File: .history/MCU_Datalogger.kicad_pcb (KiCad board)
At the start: 2 copper layers, 29 parts, among them J1 Conn_01x04_Pin, J2 Conn_01x04_Pin, J3 Conn_01x09_Pin, J4 Conn_02x03_Odd_Even, U1 24LC1025, U2 24LC1025, U3 DS1337S_, U4 ATMEGA328P-AU, Y1 32.768 KHz, Y2 16 MHz

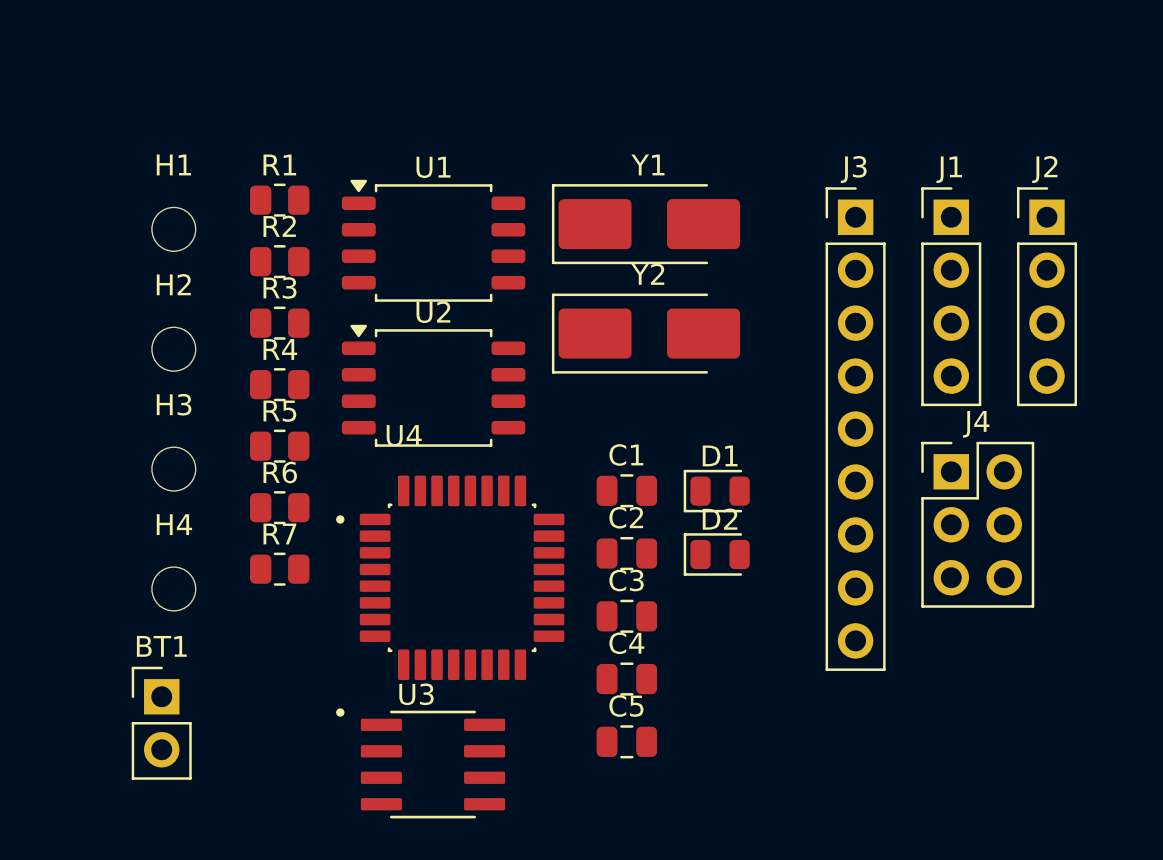
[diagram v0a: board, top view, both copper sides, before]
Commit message: footprint placement completed
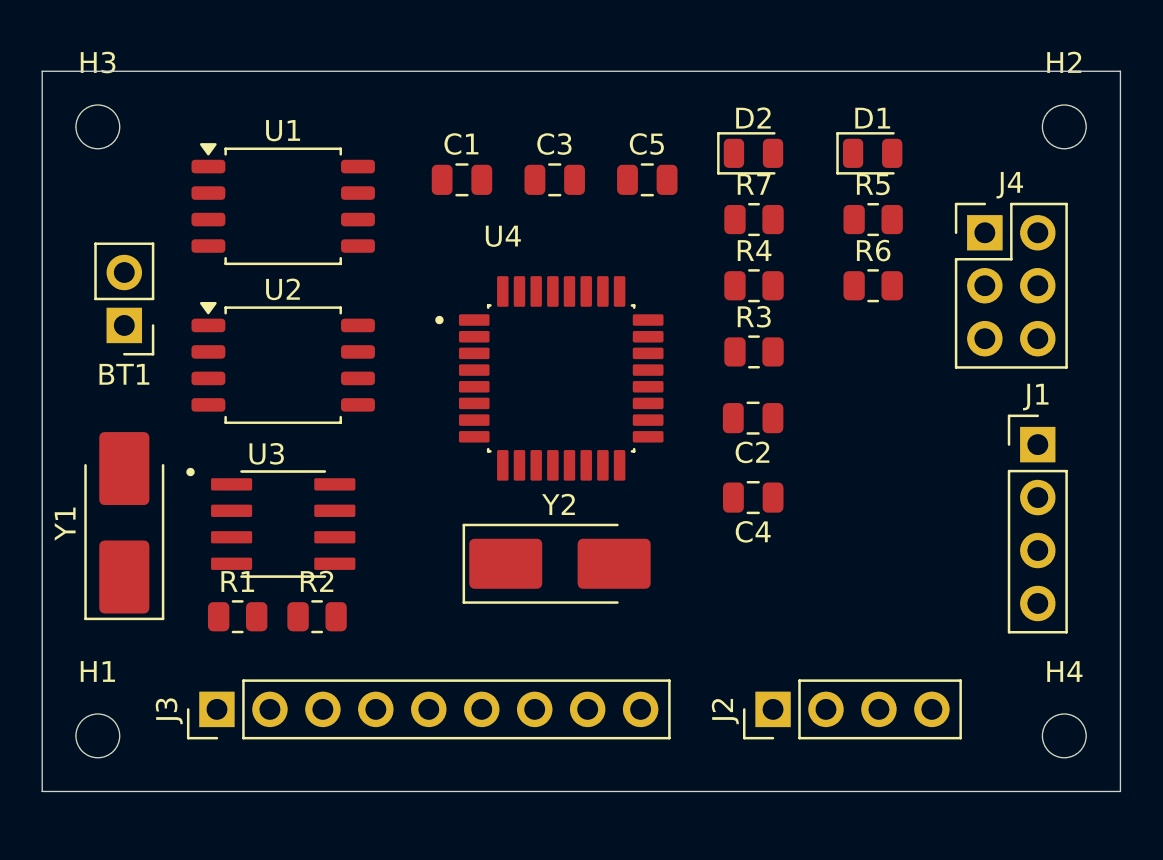
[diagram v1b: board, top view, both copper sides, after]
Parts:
- moved H2 44.0 mm to (156.2, 64.1)
- moved H4 43.3 mm to (156.2, 93.3)
- moved J3 38.7 mm to (115.6, 92.1), turned to 90 degrees
- moved R5 30.5 mm to (147.0, 68.6)
- moved R6 30.4 mm to (147.0, 71.8)
- moved Y1 29.0 mm to (111.1, 83.1), turned to 90 degrees
- moved R7 28.3 mm to (141.3, 68.6)
- moved J2 27.0 mm to (142.2, 92.1), turned to 90 degrees
- moved C5 27.0 mm to (136.2, 66.7)
- moved H1 24.6 mm to (109.9, 93.3)
- moved R4 23.2 mm to (141.3, 71.8)
- moved R3 22.8 mm to (141.3, 74.9)
- moved C3 21.2 mm to (131.8, 66.7)
- moved R1 20.1 mm to (116.6, 87.6)
- moved D2 19.3 mm to (141.3, 65.4)
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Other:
- board outline added: 51.7 x 34.5 mm
